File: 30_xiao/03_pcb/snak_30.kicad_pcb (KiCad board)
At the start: 2 copper layers, 114 x 99.6 mm, 158 parts

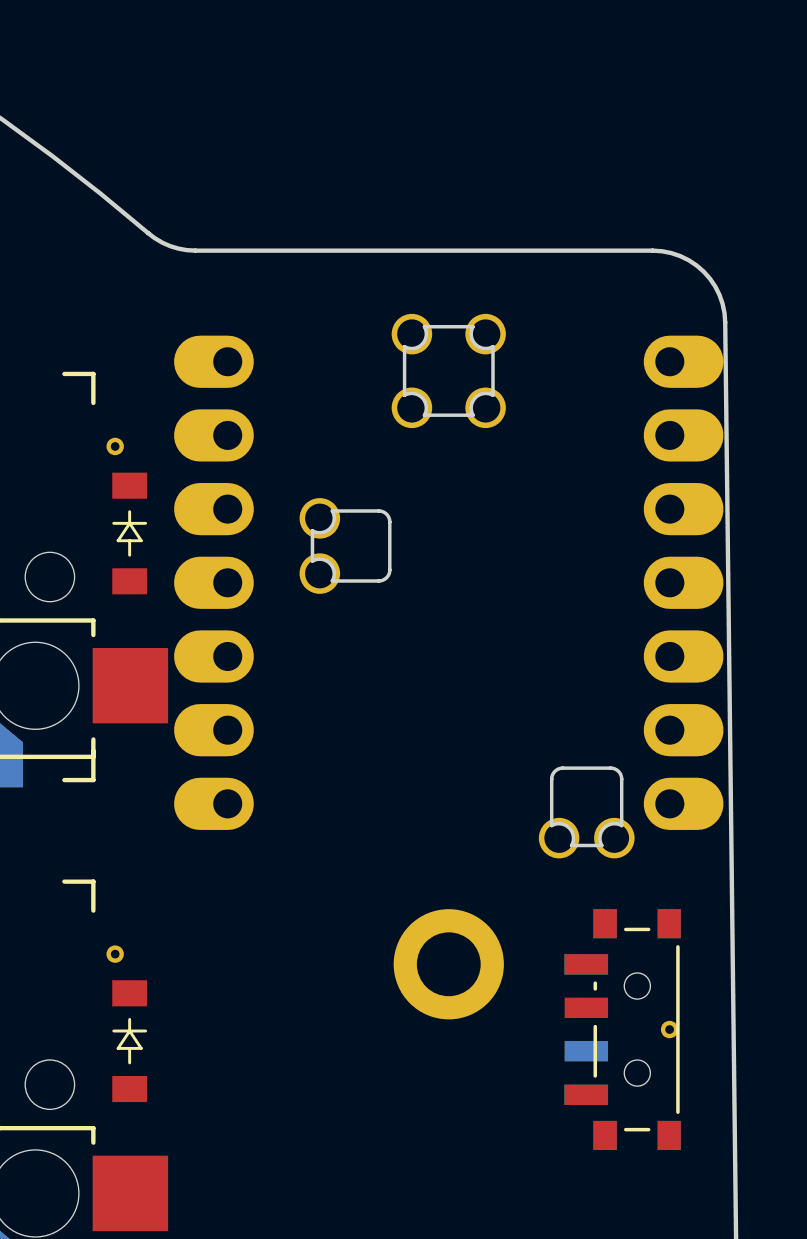
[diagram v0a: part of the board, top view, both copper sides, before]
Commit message: test xiao fp
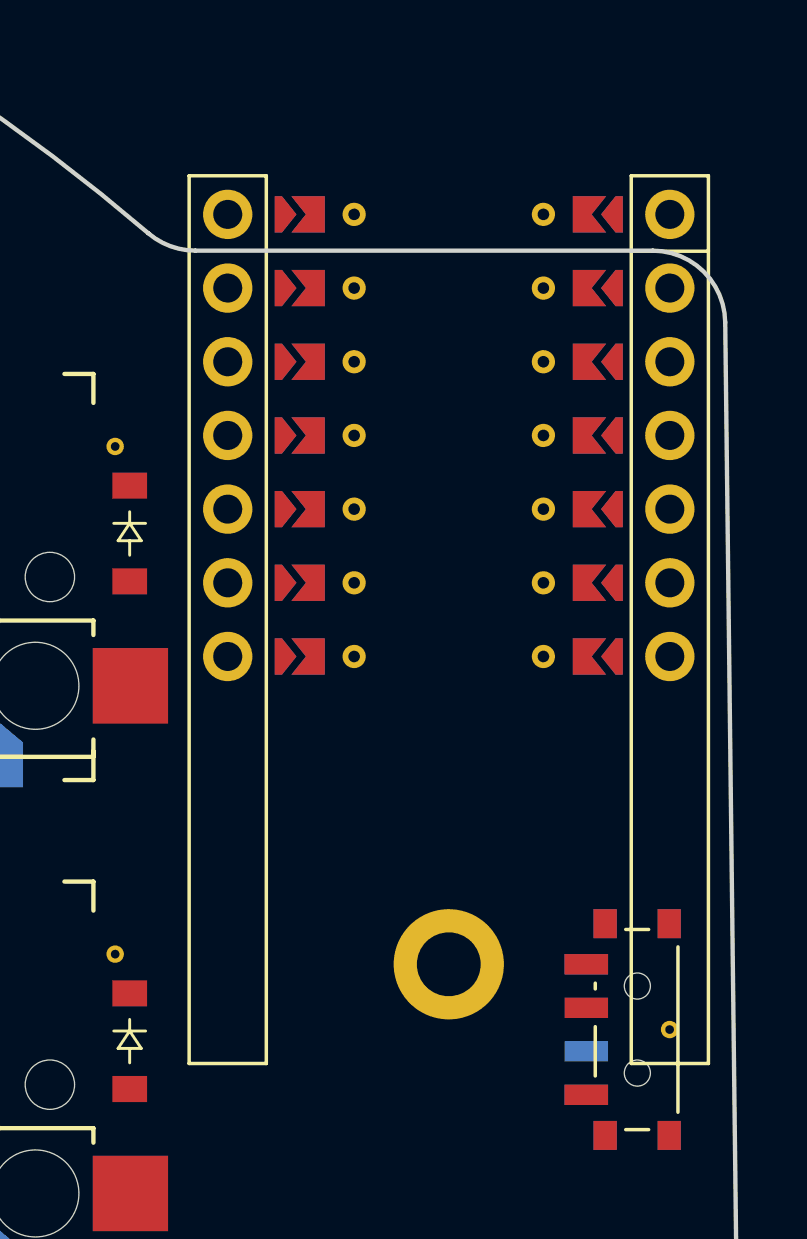
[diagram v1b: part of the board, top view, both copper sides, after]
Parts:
- MCU1: value xiao-ble -> (none); footprint XIAO-BLE -> nice_nano
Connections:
- net BAT_NEG renamed MCU1_20
- net NFC0 renamed MCU1_21
- net NFC1 renamed MCU1_22
- net RST renamed MCU1_18
- DISP1 pad 14: P10 -> DPD
- DISP1 pad 15: P8 -> DPC
- DISP1 pad 17: P9 -> DPE
- DISP1 pad 24: P10 -> DPD
- DISP1 pad 25: P8 -> DPC
- DISP1 pad 27: P9 -> DPE
- MCU1 pad 1: C1 -> MCU1_1
- MCU1 pad 19: BAT_POS -> MCU1_19
- MCU1 pad 2: C2 -> MCU1_2
- MCU1 pad 3: C3 -> MCU1_3
- MCU1 pad 4: C4 -> MCU1_4
- MCU1 pad 5: C5 -> MCU1_5
- MCU1 pad 6: P5 -> MCU1_6
- MCU1 pad 7: P6 -> MCU1_7
